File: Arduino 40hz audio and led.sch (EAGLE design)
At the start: 28 parts, among them IC1 LM7805, IC2 IRL-Z44N, IC3 LM741

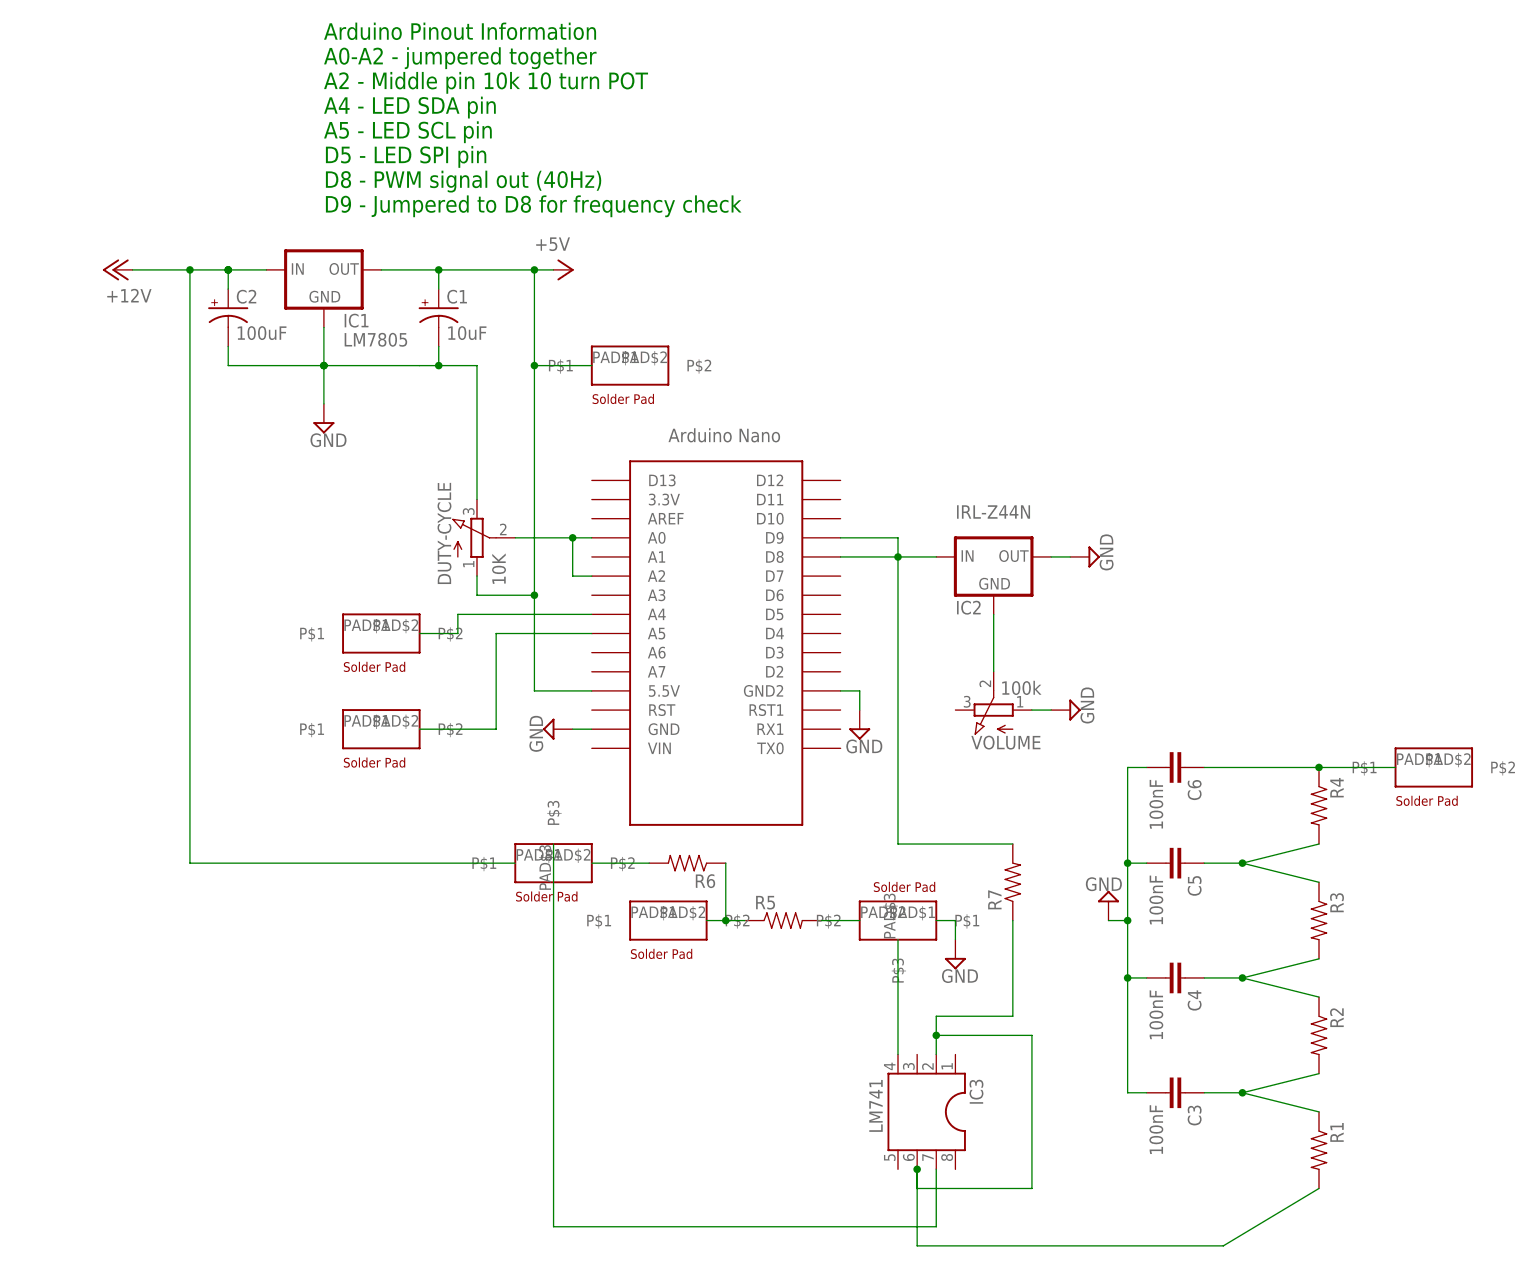
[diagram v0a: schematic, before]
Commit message: Version 1 is done.. w00t
Version 1 is done.. w00t!!!

Now I need to make some little fixes as I've built the first one.
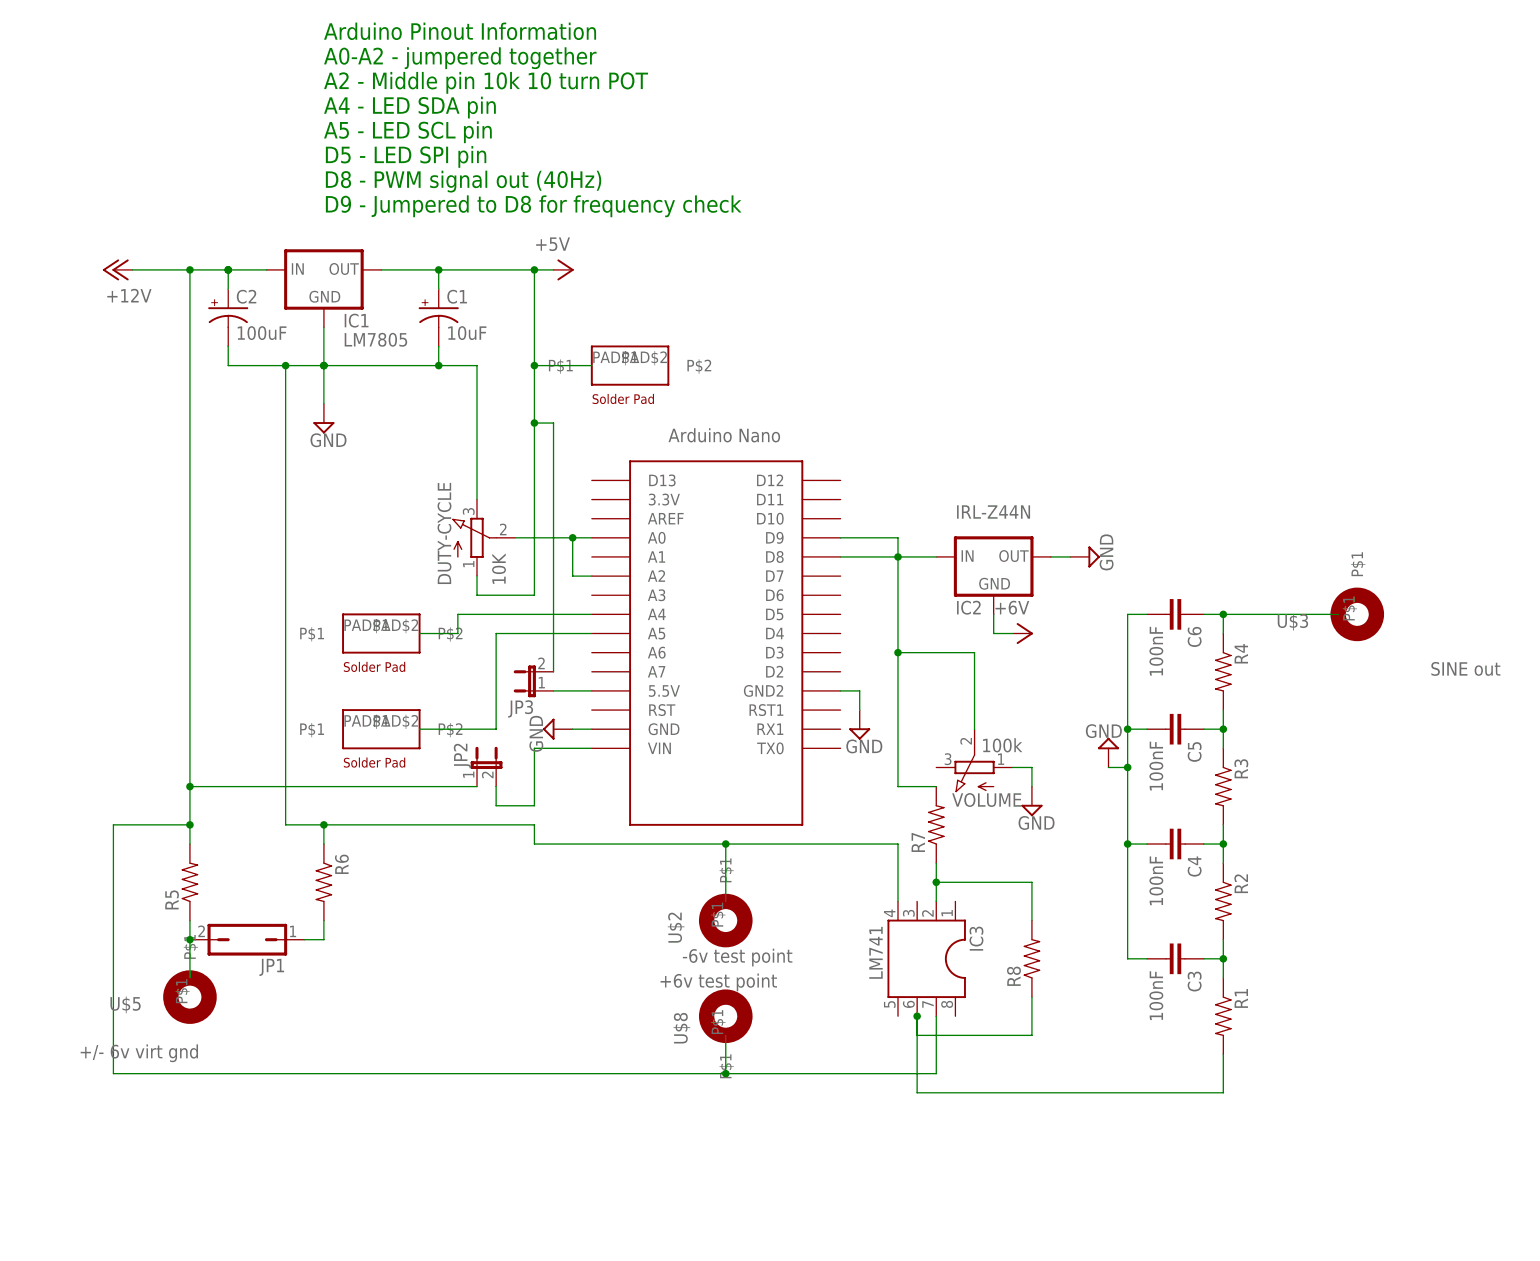
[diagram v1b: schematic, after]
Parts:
- added JP1: (no value), jumper:JP1Q
- added JP2, JP3: (no value), jim_muppet_parts:JUMPER-JP1E
- added P+3: +6V, jim_muppet_parts:+6V
- added R8: (no value), jim_muppet_parts:RESISTORPTH-1/4W
- U$2: value PAD-2PIN-RECTANGLE -> -6v test point; device jim_muppet_parts:PAD-2PIN-RECTANGLE -> jim_muppet_parts:PROBE-POINTPROBE_POINT_1
- U$3: value PAD-3PIN-RECTANGLE50MIL -> SINE out; device jim_muppet_parts:PAD-3PIN-RECTANGLE50MIL -> jim_muppet_parts:PROBE-POINTPROBE_POINT_1
- U$5: value PAD-3PIN-RECTANGLE50MIL -> +/- 6v virt gnd; device jim_muppet_parts:PAD-3PIN-RECTANGLE50MIL -> jim_muppet_parts:PROBE-POINTPROBE_POINT_1
- U$8: value PAD-2PIN-RECTANGLE -> +6v test point; device jim_muppet_parts:PAD-2PIN-RECTANGLE -> jim_muppet_parts:PROBE-POINTPROBE_POINT_1
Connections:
- removed net N$11: IC3.7, U$5.P$3
- removed net N$12: IC3.4, U$3.P$3
- new net N$16: JP1.2, R5.1, U$5.P$1
- net +12V: now also IC3.7, JP2.1, R5.2, U$8.P$1; no longer U$5.P$1
- net +5V: now also IC2.GND, JP3.2, P+3.+5V; no longer U$1.5.5V
- net GND: now also IC3.4, R6.1, U$2.P$1; no longer U$3.P$1
- net N$10: now also IC3.2, R7.1, R8.2; no longer R5.2, U$3.P$2
- net N$13: now also R8.1; no longer IC3.2, R7.1
- net N$2: now also VOLUME.S
- net N$6: no longer U$2.P$1
- net N$7: now also JP1.1; no longer U$5.P$2
- net N$8: now also JP2.2, U$1.VIN; no longer IC2.GND, VOLUME.S
- net N$9: now also JP3.1, U$1.5.5V; no longer R5.1, R6.1, U$8.P$2
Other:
- moved on the sheet: C3, C4, C5, C6, IC3, R1, R2, R3, R4, R5, R6, R7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
